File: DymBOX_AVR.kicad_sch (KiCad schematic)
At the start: 37 parts, among them J1 Conn_01x04_Pin, J3 Conn_01x02_Pin, J4 DS18B20, J5 Conn_02x05_Odd_Even, Q1 BC327, Q2 BC327, Q3 BS170, Q4 BS170, Q5 BC327, SW1 RotaryEncoder_Switch, U1 ATmega8A-P, U2 CA56-12EWA, U3 L7805, Y1 Crystal

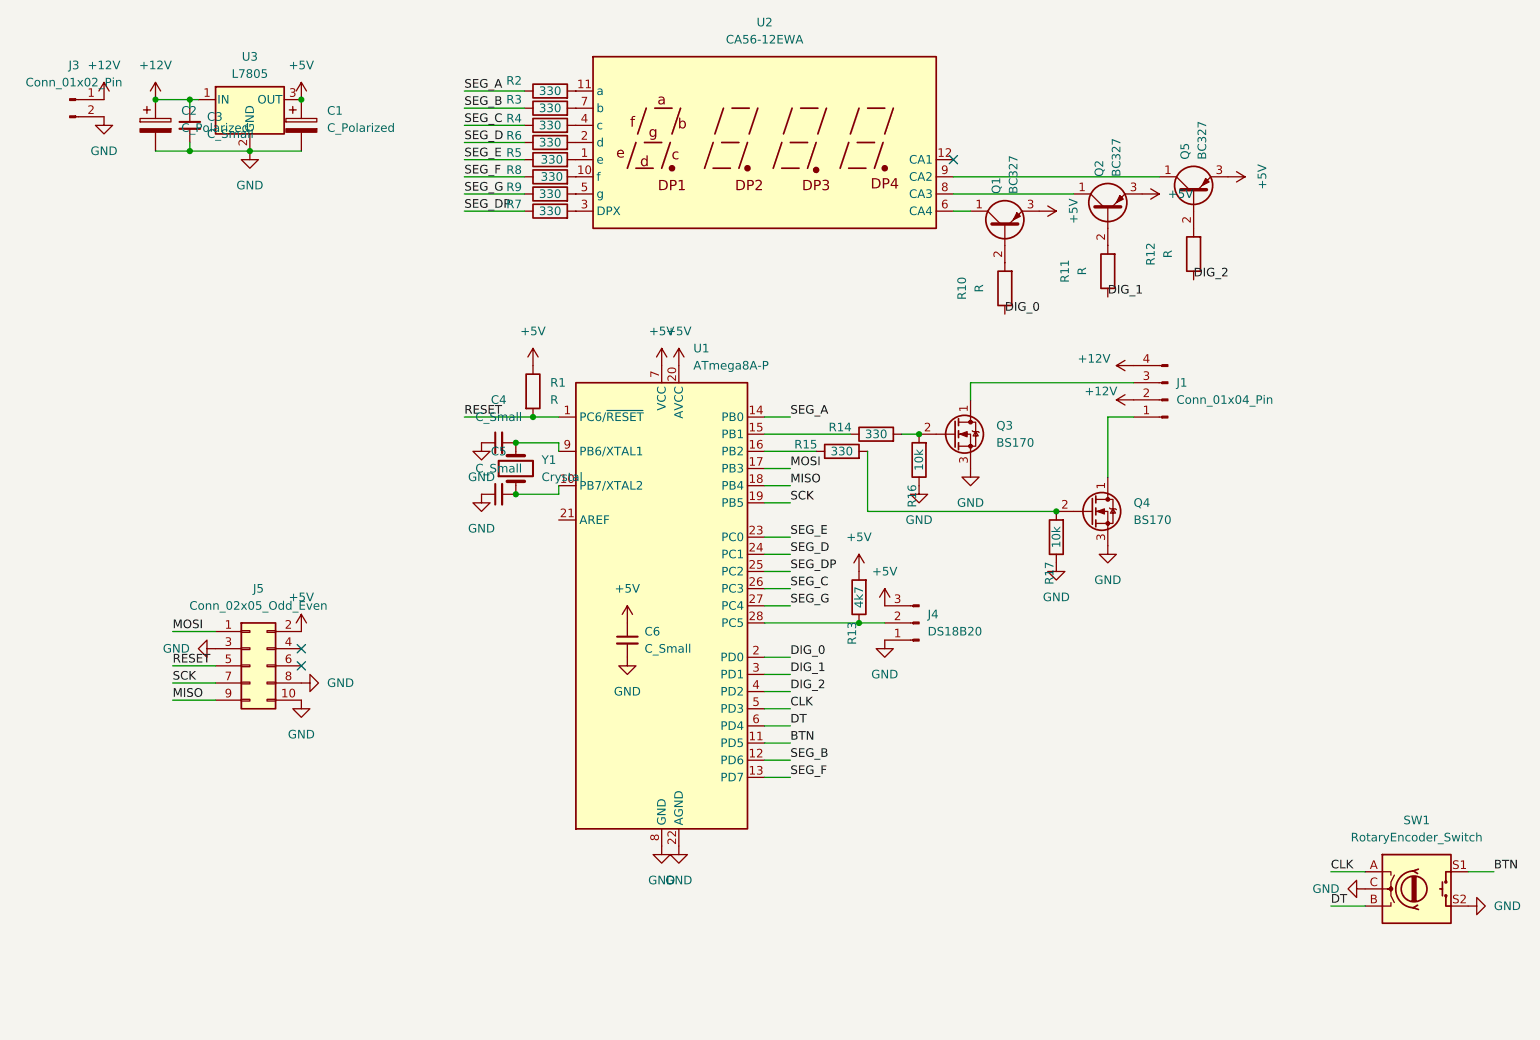
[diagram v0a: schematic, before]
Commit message: pcb_transfo
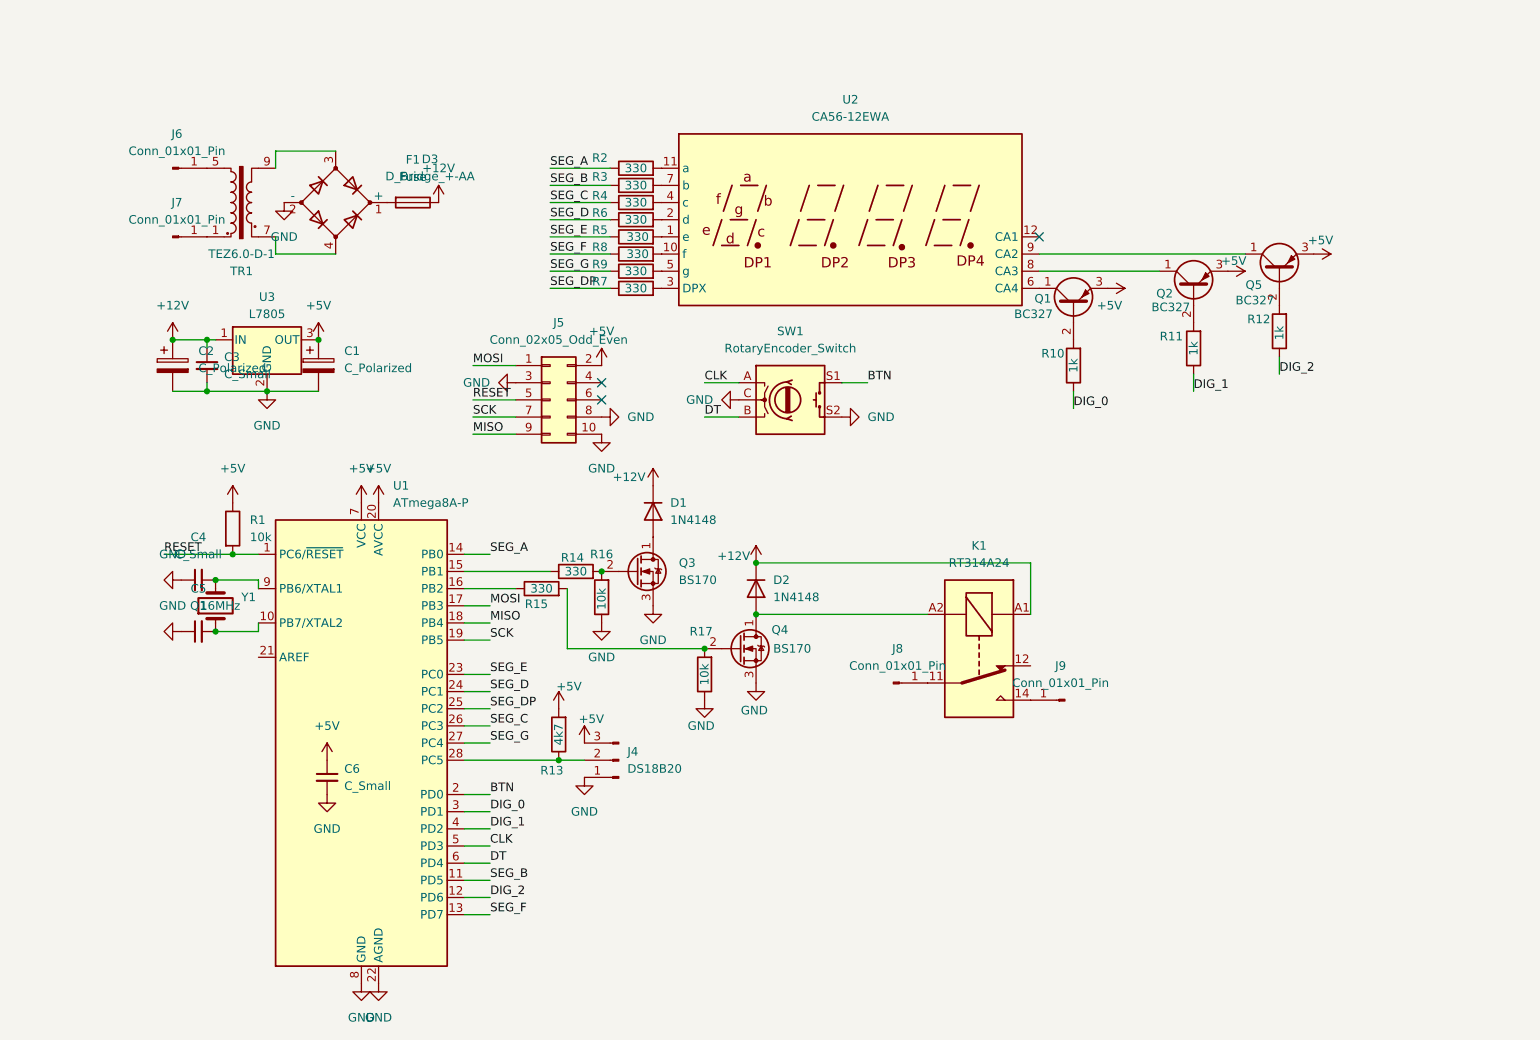
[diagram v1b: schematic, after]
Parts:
- removed J1: Conn_01x04_Pin, Connector_Phoenix_MC:PhoenixContact_MCV_1,5_4-G-3.5_1x04_P3.50mm_Vertical, symbol Connector:Conn_01x04_Pin
- removed J3: Conn_01x02_Pin, Connector_Phoenix_MC:PhoenixContact_MCV_1,5_2-G-3.5_1x02_P3.50mm_Vertical, symbol Connector:Conn_01x02_Pin
- added D1, D2: 1N4148, Diode_THT:D_DO-35_SOD27_P7.62mm_Horizontal, symbol Diode:1N4148
- added D3: D_Bridge_+-AA, Diode_THT:Diode_Bridge_DIP-4_W5.08mm_P2.54mm, symbol Device:D_Bridge_+-AA
- added F1: Fuse, Fuse:Fuseholder_Clip-5x20mm_Littelfuse_111_Inline_P20.00x5.00mm_D1.05mm_Horizontal, symbol Device:Fuse
- added J6, J7, J8, J9: Conn_01x01_Pin, 2pkstartup:TRM2_62409-1_TEC, symbol 2pkstartup:FST
- added K1: RT314A24, Relay_THT:Relay_SPDT_Schrack-RT1-16A-FormC_RM5mm, symbol Relay:RT314A24
- added TR1: TEZ6.0-D-1, Transformer_THT:Transformer_Breve_TEZ-38x45, symbol Transformer:TEZ6.0-D-1
- C1, C2: footprint Capacitor_THT:CP_Radial_D10.0mm_P7.50mm -> Capacitor_THT:CP_Radial_D13.0mm_P5.00mm
- C5: value C_Small -> Q1
- J4: footprint Connector_Phoenix_MC:PhoenixContact_MCV_1,5_3-G-3.5_1x03_P3.50mm_Vertical -> Connector_Wire:SolderWire-0.127sqmm_1x03_P3.7mm_D0.48mm_OD1mm
- Q1: footprint Package_TO_SOT_THT:TO-92L_HandSolder -> Package_TO_SOT_THT:TO-92_HandSolder
- Q3, Q4: footprint Package_TO_SOT_THT:TO-92_Inline -> Package_TO_SOT_THT:TO-92_HandSolder
- R1: value R -> 10k
- R10, R11, R12: value R -> 1k
- Y1: value Crystal -> 16MHz
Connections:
- net +12V: now also D1.1 (K), D2.1 (K), F1.1, K1.A1
- net BTN: now also U1.2 (PD0); no longer U1.11 (PD5)
- net DIG_0: now also U1.3 (PD1); no longer U1.2 (PD0)
- net DIG_1: now also U1.4 (PD2); no longer U1.3 (PD1)
- net DIG_2: now also U1.12 (PD6); no longer U1.4 (PD2)
- net GND: now also D3.2 (-)
- net SEG_B: now also U1.11 (PD5); no longer U1.12 (PD6)
- net at Q3.1 (D): now also D1.2 (A)
- net at Q4.1 (D): now also D2.2 (A), K1.A2
- new net: D3.1 (+), F1.2
- new net: J8.1 (Pin_1), K1.11
- new net: J6.1 (Pin_1), TR1.5
- new net: D3.3, TR1.9
- new net: D3.4, TR1.7
- new net: J7.1 (Pin_1), TR1.1
- new net: J9.1 (Pin_1), K1.14
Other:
- moved on the sheet: C1, C2, C3, C4, C5, C6, J4, J5, Q1, Q2, Q3, Q4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
